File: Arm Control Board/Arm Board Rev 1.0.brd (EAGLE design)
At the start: 189.8 x 119.2 mm, 54 parts

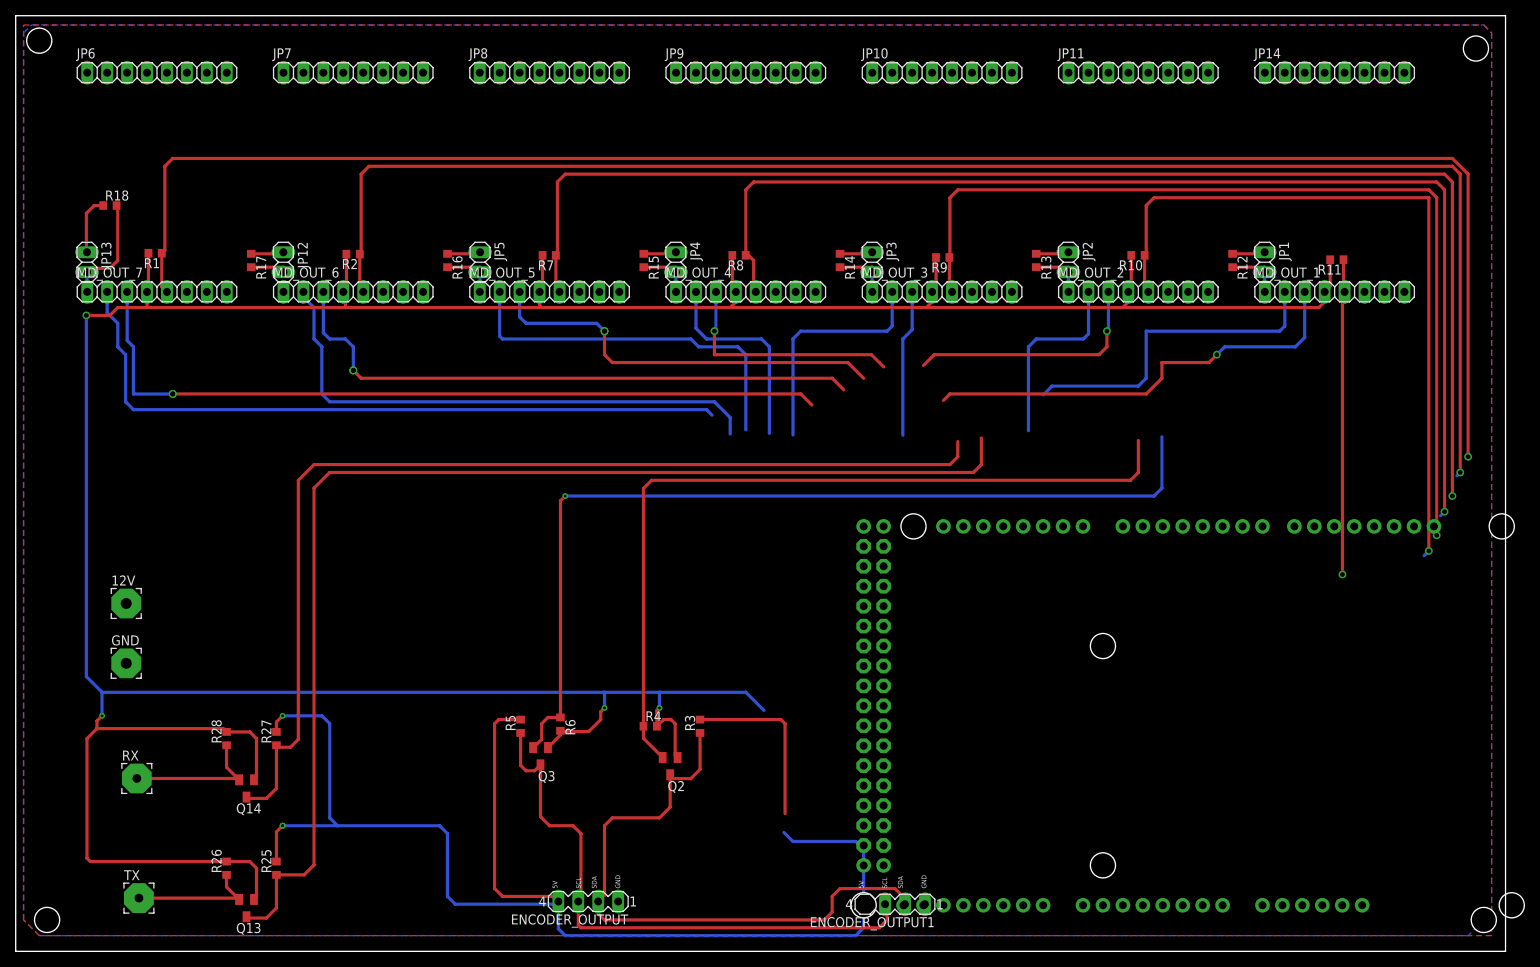
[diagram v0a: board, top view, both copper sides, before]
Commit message: test
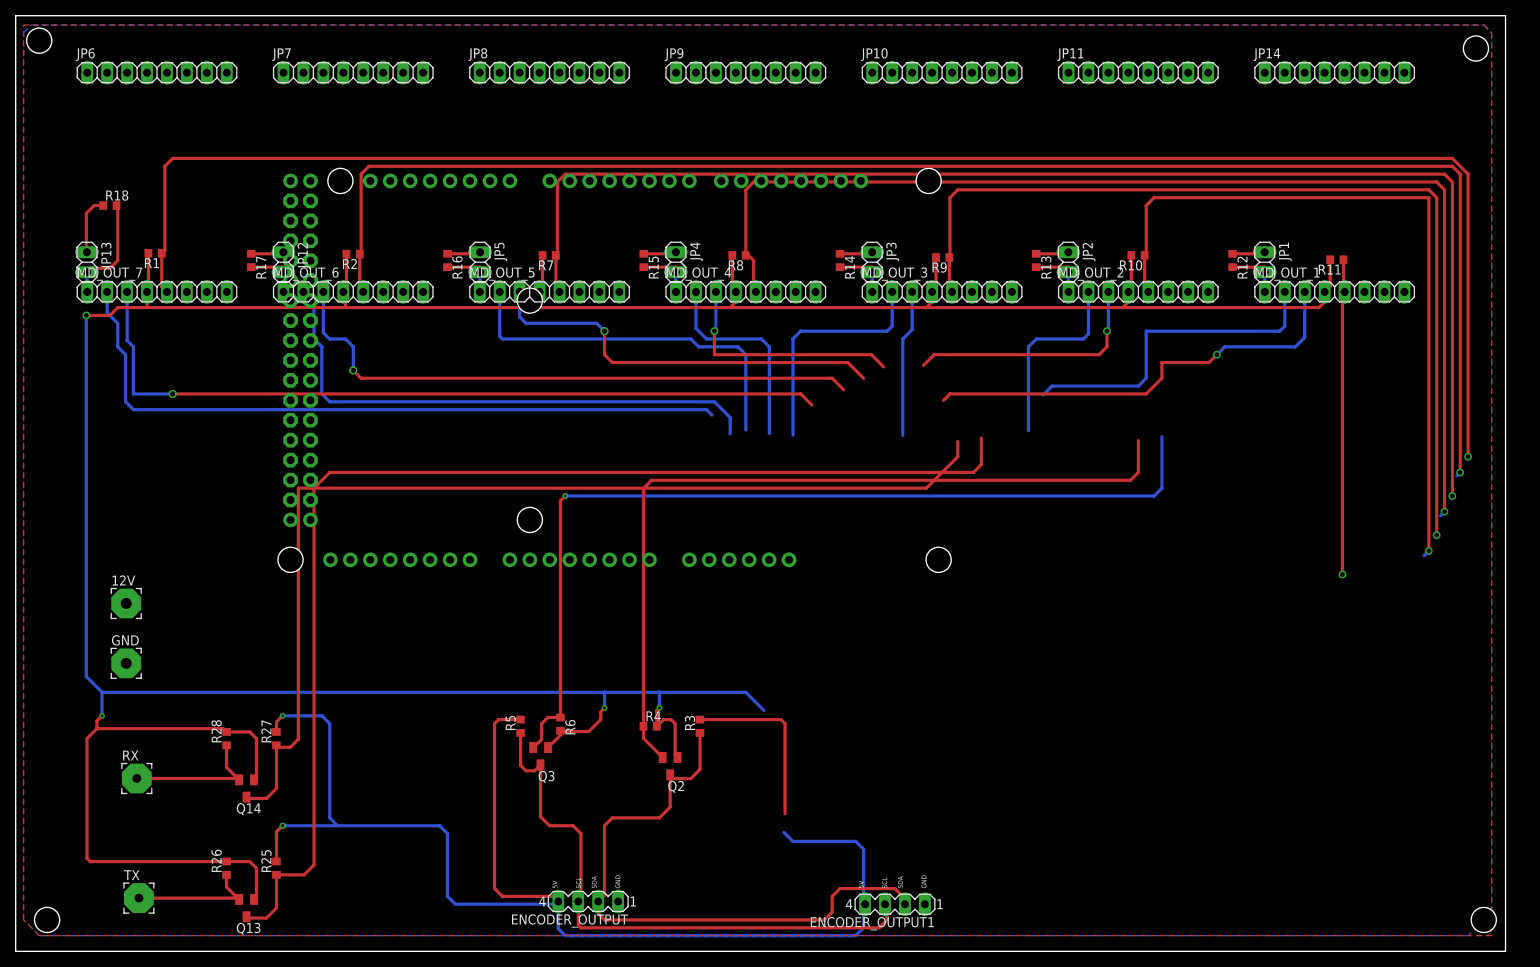
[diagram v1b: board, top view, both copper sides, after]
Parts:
- moved B1 85.2 mm to (78.0, 74.0)
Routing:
- net TX: track 133.4 -> 132.8 mm
